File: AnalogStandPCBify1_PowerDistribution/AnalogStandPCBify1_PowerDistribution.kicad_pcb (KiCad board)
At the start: 2 copper layers, 13 parts, among them SW1 SOL_SW, SW2 SOL_SW, SW3 SOL_SW, SW4 SOL_SW

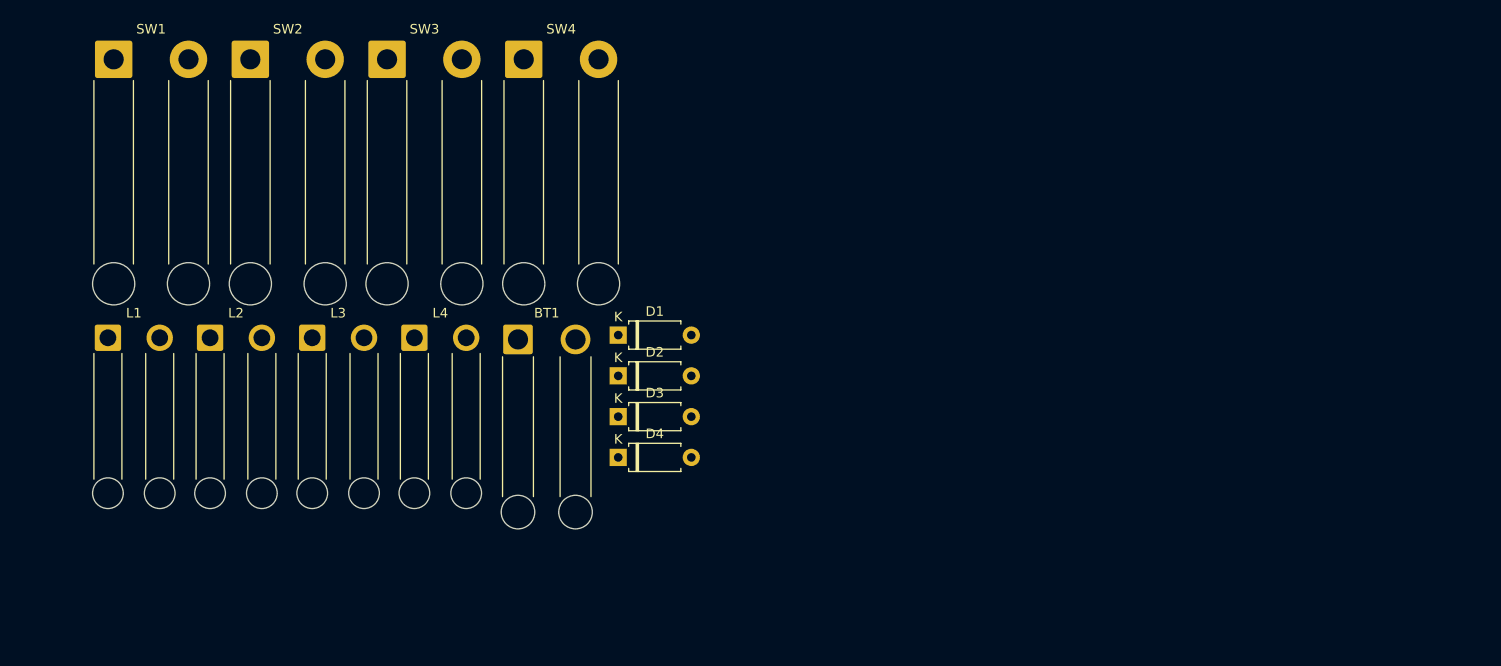
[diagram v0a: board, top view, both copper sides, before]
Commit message: Push
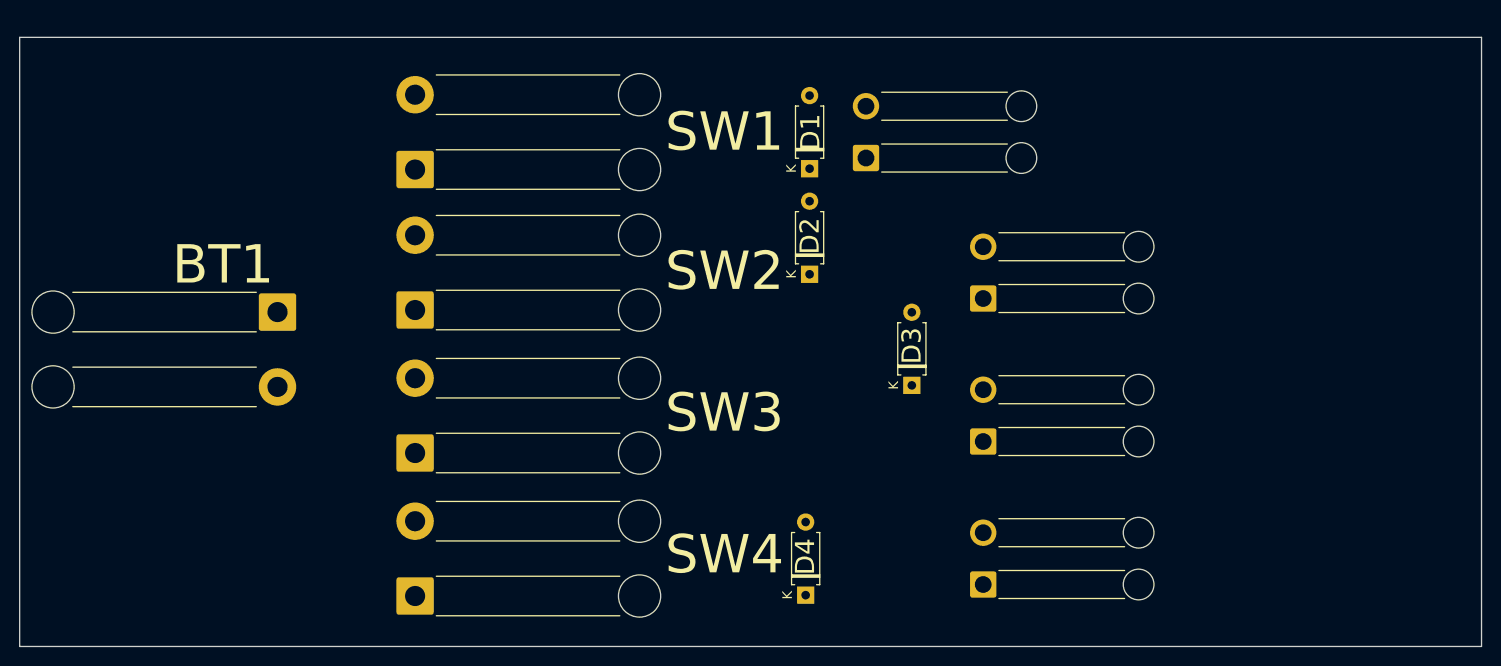
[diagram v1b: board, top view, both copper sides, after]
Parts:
- BT1: footprint Connector_Wire:SolderWire-1.5sqmm_1x02_P6mm_D1.7mm_OD3mm_Relief -> Connector_Wire:SolderWire-1.5sqmm_1x02_P7.8mm_D1.7mm_OD3.9mm_Relief
- moved L1 81.2 mm to (113.6, 38.0), turned to 90 degrees
- moved L2 80.7 mm to (125.8, 52.6), turned to 90 degrees
- moved L3 70.8 mm to (125.8, 67.5), turned to 90 degrees
- moved L4 64.6 mm to (125.8, 82.4), turned to 90 degrees
- moved SW4 57.1 mm to (66.6, 83.6), turned to 90 degrees
- moved SW3 41.1 mm to (66.6, 68.7), turned to 90 degrees
- moved SW1 33.5 mm to (66.6, 39.2), turned to 90 degrees
- moved SW2 31.3 mm to (66.6, 53.8), turned to 90 degrees
- moved D3 30.8 mm to (118.4, 61.7), turned to 90 degrees
- moved D1 26.4 mm to (107.8, 39.1), turned to 90 degrees
- moved BT1 25.2 mm to (52.3, 54.0), turned to -90 degrees
- moved D4 24.2 mm to (107.3, 83.5), turned to 90 degrees
- moved D2 22.6 mm to (107.8, 50.1), turned to 90 degrees
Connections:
- net Net-(BT1-+) renamed /24V+
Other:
- board outline added: 152.4 x 63.5 mm

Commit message: A
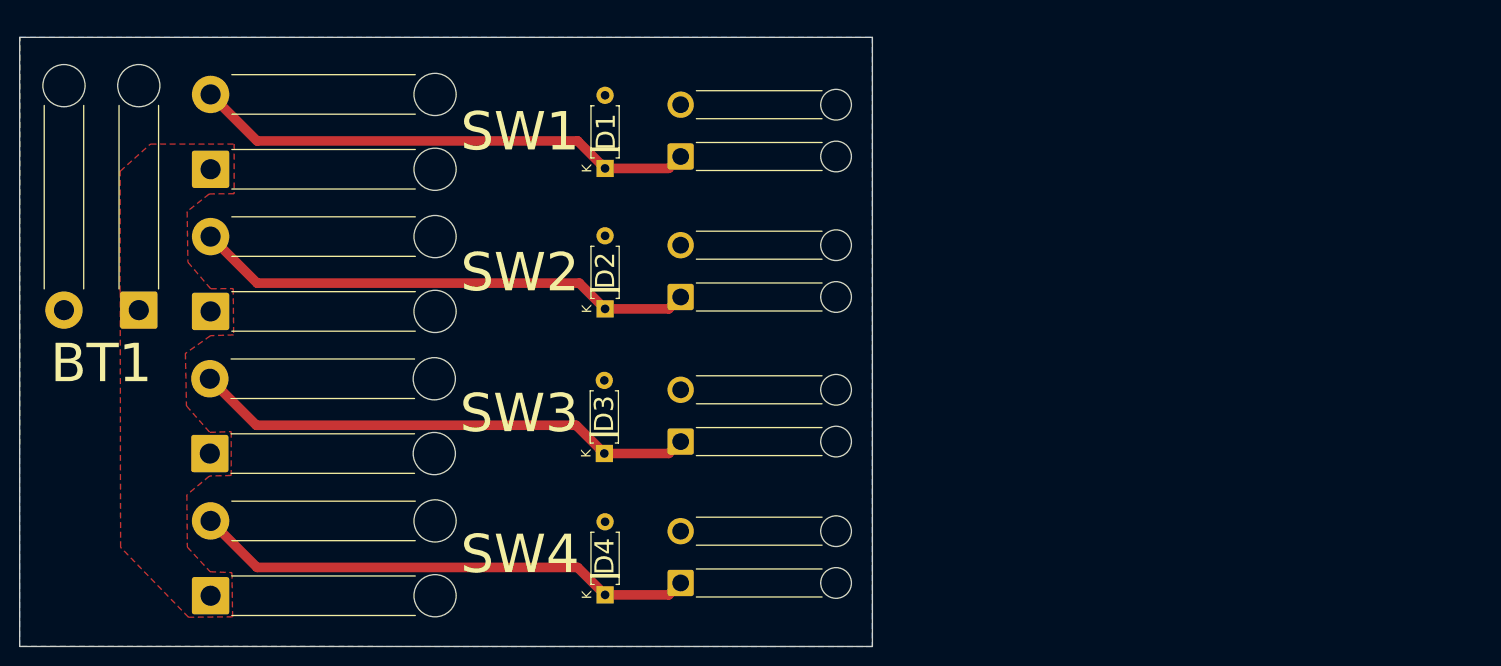
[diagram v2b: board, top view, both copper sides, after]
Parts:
- moved D3 32.8 mm to (86.3, 68.8)
- moved L2 31.5 mm to (94.3, 52.5)
- moved L4 31.5 mm to (94.3, 82.3)
- moved L3 31.5 mm to (94.3, 67.5)
- moved D2 21.6 mm to (86.4, 53.7)
- moved SW3 21.4 mm to (45.2, 68.8)
- moved SW2 21.3 mm to (45.3, 54.0)
- moved SW1 21.3 mm to (45.3, 39.1)
- moved SW4 21.3 mm to (45.3, 83.6)
- moved D1 21.3 mm to (86.4, 39.1)
- moved D4 20.9 mm to (86.4, 83.5)
- moved L1 19.3 mm to (94.3, 37.8)
- moved BT1 14.5 mm to (37.8, 53.8), turned to 180 degrees
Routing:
- net Net-(D3-K): track 0.00 -> 52.8 mm
- net Net-(D1-K): track 0.00 -> 52.7 mm
- net Net-(D4-K): track 0.00 -> 52.7 mm
- net Net-(D2-K): track 0.00 -> 52.6 mm
- added copper zone on F.Cu, net /24V+
- added copper zone on B.Cu, net GND
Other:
- board size 152.4 x 63.5 mm -> 88.9 x 63.5 mm
